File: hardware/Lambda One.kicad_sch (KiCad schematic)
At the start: 5 parts, among them IC1 01, SW1 SW_Push, U1 W65C816SxP, U3 ATF22V10C, Y1 TFT680

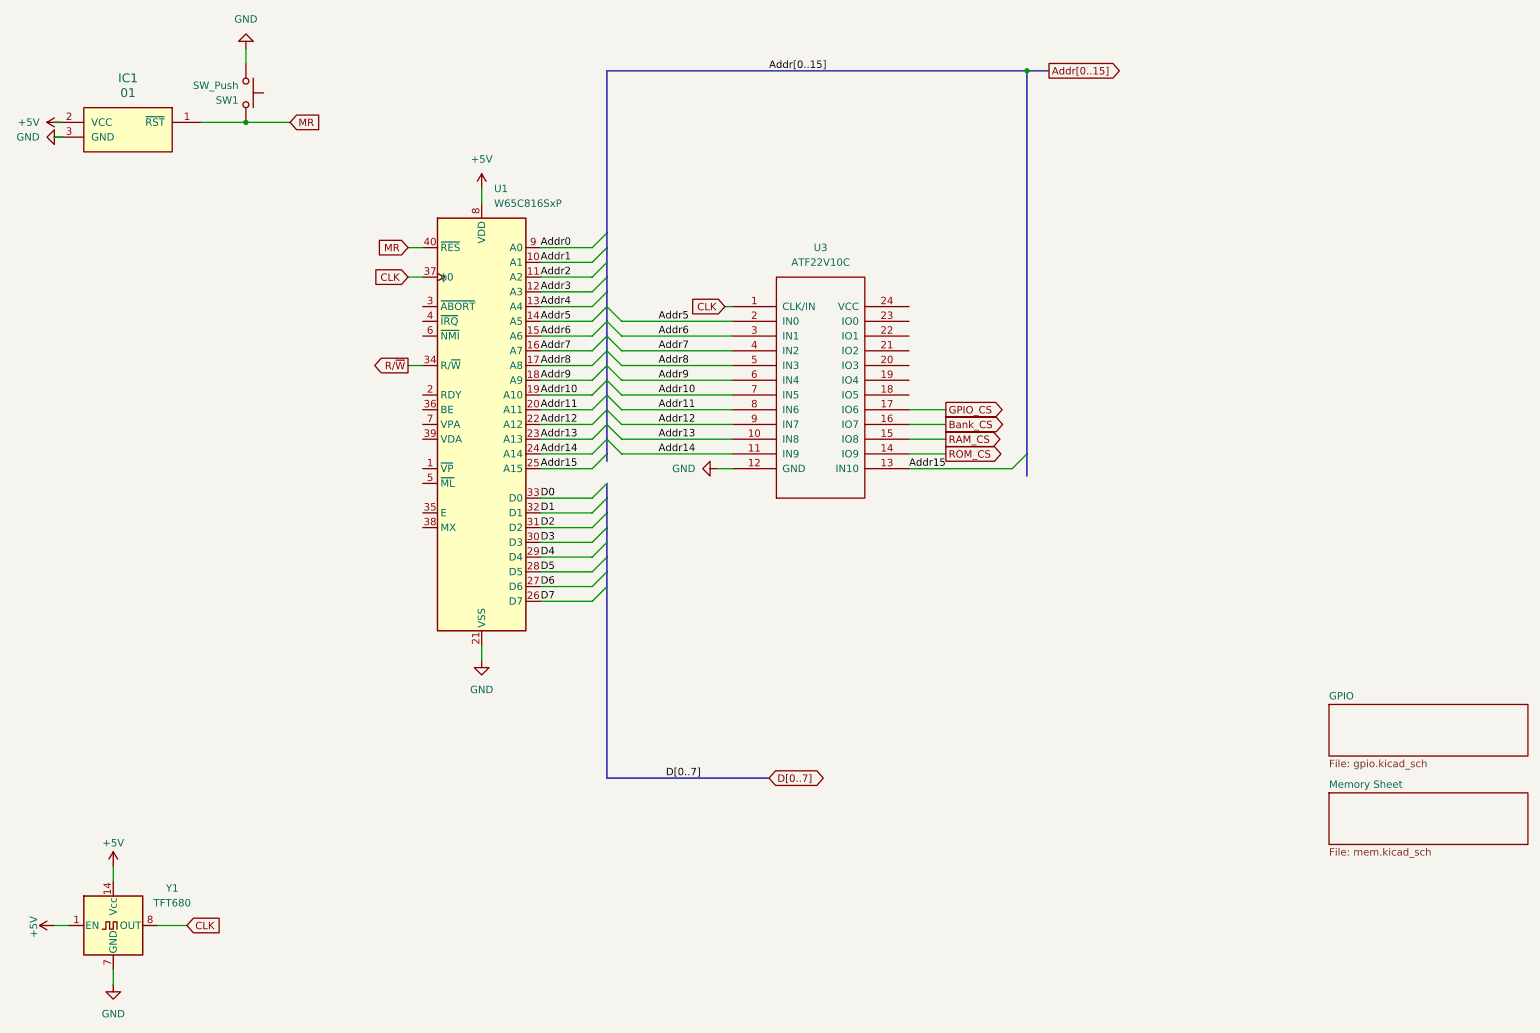
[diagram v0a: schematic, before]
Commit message: Improved labels
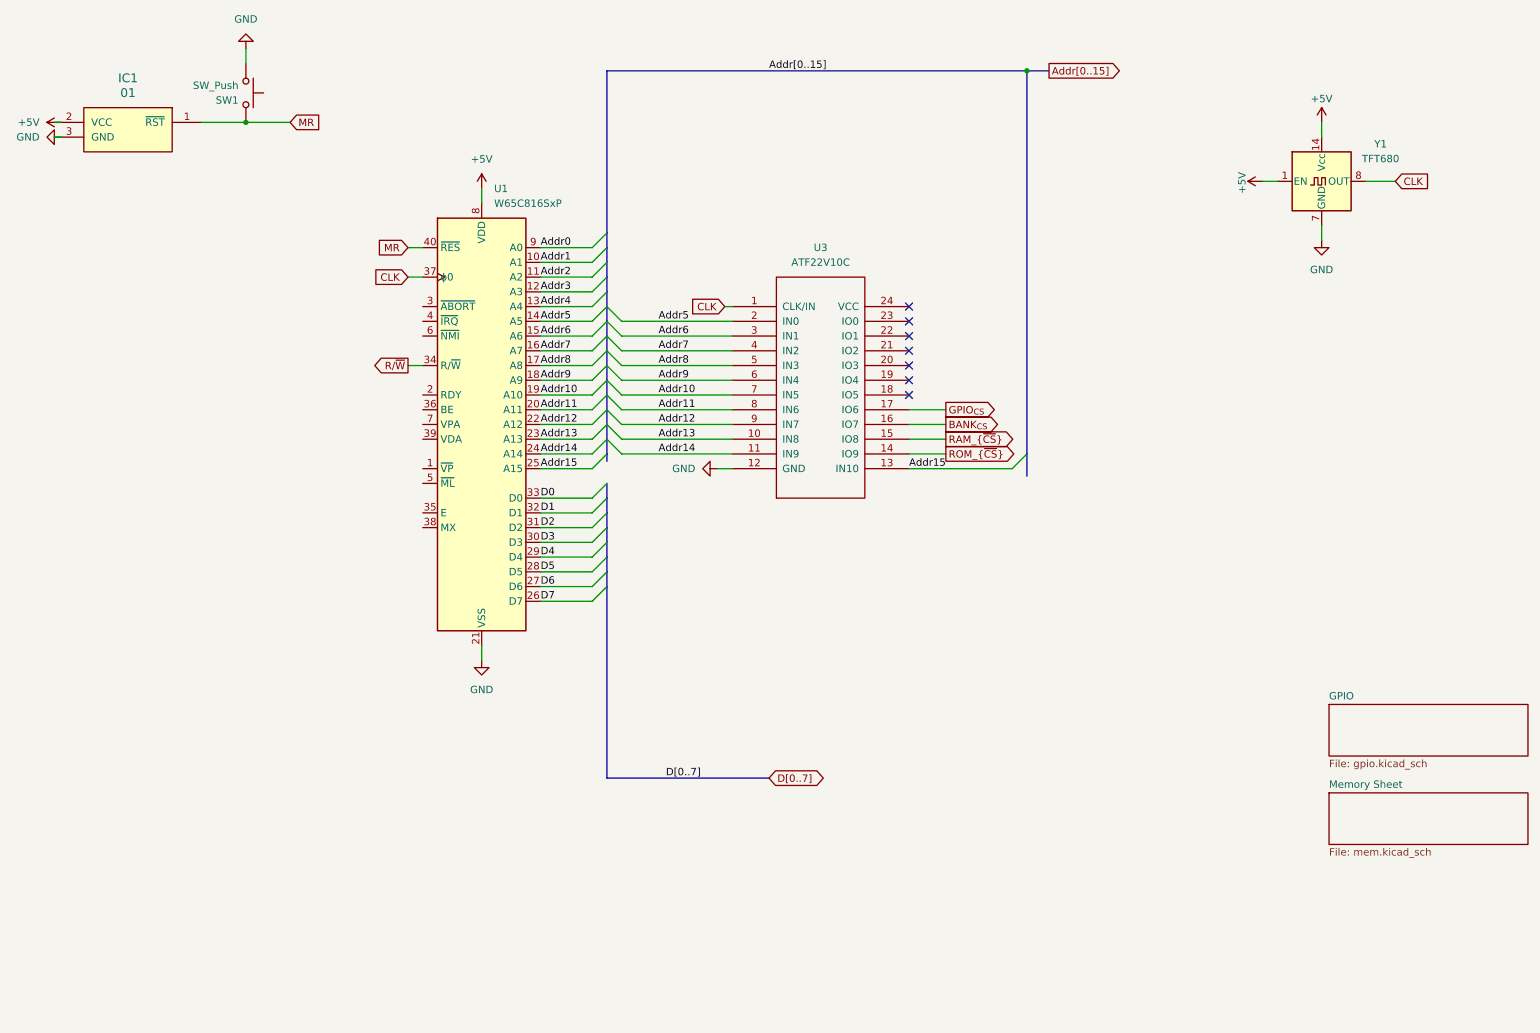
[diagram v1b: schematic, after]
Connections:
- net Bank_CS renamed BANK_{CS}
- net GPIO_CS renamed GPIO_{CS}
- net RAM_CS renamed RAM_{~{CS}}
- net ROM_CS renamed ROM_{~{CS}}
- no-connect marks 0 -> 7
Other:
- moved on the sheet: Y1
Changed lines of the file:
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@@
 		(color 0 0 0 0)
+	)
+	(no_connect
+		(at 175.26 69.85)
+	)
+	(no_connect
+		(at 175.26 72.39)
+	)
+	(no_connect
+		(at 175.26 77.47)
+	)
+	(no_connect
+		(at 175.26 82.55)
+	)
+	(no_connect
+		(at 175.26 85.09)
+	)
+	(no_connect
+		(at 175.26 80.01)
+	)
+	(no_connect
+		(at 175.26 74.93)
 	)
 	(bus_entry
@@
 	(wire
 		(pts
-			(xy 38.1 184.15) (xy 38.1 186.69)
+			(xy 246.38 55.88) (xy 246.38 58.42)
 		)
 		(stroke
@@
 	(wire
 		(pts
-			(xy 27.94 176.53) (xy 30.48 176.53)
+			(xy 236.22 48.26) (xy 238.76 48.26)
 		)
 		(stroke
@@
 	(wire
 		(pts
-			(xy 38.1 166.37) (xy 38.1 168.91)
+			(xy 246.38 38.1) (xy 246.38 40.64)
 		)
 		(stroke
@@
 	(wire
 		(pts
-			(xy 45.72 176.53) (xy 50.8 176.53)
+			(xy 254 48.26) (xy 259.08 48.26)
 		)
 		(stroke
@@
 	(global_label "CLK"
 		(shape input)
-		(at 50.8 176.53 0)
+		(at 259.08 48.26 0)
 		(fields_autoplaced yes)
 		(effects
@@
 		)
 		(property "Intersheetrefs" "${INTERSHEET_REFS}"
-			(at 57.3533 176.53 0)
+			(at 265.6333 48.26 0)
 			(effects
 				(font
@@
 		)
 	)
-	(global_label "ROM_CS"
+	(global_label "ROM_{~{CS}}"
 		(shape output)
 		(at 181.61 95.25 0)
@@
 		)
 		(property "Intersheetrefs" "${INTERSHEET_REFS}"
-			(at 192.0942 95.25 0)
+			(at 190.6815 95.25 0)
 			(effects
 				(font
@@
 		)
 	)
-	(global_label "Bank_CS"
+	(global_label "BANK_{CS}"
 		(shape output)
 		(at 181.61 90.17 0)
@@
 		)
 		(property "Intersheetrefs" "${INTERSHEET_REFS}"
-			(at 192.6384 90.17 0)
+			(at 191.5887 90.17 0)
 			(effects
 				(font
@@
 		)
 	)
-	(global_label "RAM_CS"
+	(global_label "RAM_{~{CS}}"
 		(shape output)
 		(at 181.61 92.71 0)
@@
 		)
 		(property "Intersheetrefs" "${INTERSHEET_REFS}"
-			(at 191.8523 92.71 0)
+			(at 190.4396 92.71 0)
 			(effects
 				(font
@@
 		)
 	)
-	(global_label "GPIO_CS"
+	(global_label "GPIO_{CS}"
 		(shape output)
 		(at 181.61 87.63 0)
@@
 		)
 		(property "Intersheetrefs" "${INTERSHEET_REFS}"
-			(at 192.5176 87.63 0)
+			(at 191.1049 87.63 0)
 			(effects
 				(font
@@
 	(symbol
 		(lib_id "power:+5V")
-		(at 27.94 176.53 90)
+		(at 236.22 48.26 90)
 		(unit 1)
 		(exclude_from_sim no)
@@
 		(dnp no)
 		(property "Reference" "#PWR020"
-			(at 31.75 176.53 0)
+			(at 240.03 48.26 0)
 			(effects
 				(font
@@
 		)
 		(property "Value" "+5V"
-			(at 24.384 176.784 0)
+			(at 232.664 48.514 0)
 			(effects
 				(font
@@
 		)
 		(property "Footprint" ""
-			(at 27.94 176.53 0)
+			(at 236.22 48.26 0)
 			(effects
 				(font
@@
 		)
 		(property "Datasheet" ""
-			(at 27.94 176.53 0)
+			(at 236.22 48.26 0)
 			(effects
 				(font
@@
 		)
 		(property "Description" "Power symbol creates a global label with name \"+5V\""
-			(at 27.94 176.53 0)
+			(at 236.22 48.26 0)
 			(effects
 				(font
@@
 	(symbol
 		(lib_id "power:+5V")
-		(at 38.1 166.37 0)
+		(at 246.38 38.1 0)
 		(unit 1)
 		(exclude_from_sim no)
@@
 		(dnp no)
 		(property "Reference" "#PWR014"
-			(at 38.1 170.18 0)
+			(at 246.38 41.91 0)
 			(effects
 				(font
@@
 		)
 		(property "Value" "+5V"
-			(at 38.1 162.306 0)
+			(at 246.38 34.036 0)
 			(effects
 				(font
@@
 		)
 		(property "Footprint" ""
-			(at 38.1 166.37 0)
+			(at 246.38 38.1 0)
 			(effects
 				(font
@@
 		)
 		(property "Datasheet" ""
-			(at 38.1 166.37 0)
+			(at 246.38 38.1 0)
 			(effects
 				(font
@@
 		)
 		(property "Description" "Power symbol creates a global label with name \"+5V\""
-			(at 38.1 166.37 0)
+			(at 246.38 38.1 0)
 			(effects
 				(font
@@
 	(symbol
 		(lib_id "Oscillator:TFT680")
-		(at 38.1 176.53 0)
+		(at 246.38 48.26 0)
 		(unit 1)
 		(exclude_from_sim no)
@@
 		(fields_autoplaced yes)
 		(property "Reference" "Y1"
-			(at 48.26 170.1098 0)
+			(at 256.54 41.8398 0)
 			(effects
 				(font
@@
 		)
 		(property "Value" "TFT680"
-			(at 48.26 172.6498 0)
+			(at 256.54 44.3798 0)
 			(effects
 				(font
@@
 		)
 		(property "Footprint" "Oscillator:Oscillator_DIP-14"
-			(at 49.53 185.42 0)
+			(at 257.81 57.15 0)
 			(effects
 				(font
@@
 		)
 		(property "Datasheet" "http://cdn-reichelt.de/documents/datenblatt/B400/OSZI.pdf"
-			(at 35.56 176.53 0)
+			(at 243.84 48.26 0)
 			(effects
 				(font
@@
 		)
 		(property "Description" "Crystal Clock Oscillator, DIP14-style metal package"
-			(at 38.1 176.53 0)
+			(at 246.38 48.26 0)
 			(effects
 				(font
@@
 	(symbol
 		(lib_id "power:GND")
-		(at 38.1 186.69 0)
+		(at 246.38 58.42 0)
 		(unit 1)
 		(exclude_from_sim no)
@@
 		(fields_autoplaced yes)
 		(property "Reference" "#PWR019"
-			(at 38.1 193.04 0)
+			(at 246.38 64.77 0)
 			(effects
 				(font
@@
 		)
 		(property "Value" "GND"
-			(at 38.1 191.77 0)
+			(at 246.38 63.5 0)
 			(effects
 				(font
@@
 		)
 		(property "Footprint" ""
-			(at 38.1 186.69 0)
+			(at 246.38 58.42 0)
 			(effects
 				(font
@@
 		)
 		(property "Datasheet" ""
-			(at 38.1 186.69 0)
+			(at 246.38 58.42 0)
 			(effects
 				(font
@@
 		)
 		(property "Description" "Power symbol creates a global label with name \"GND\" , ground"
-			(at 38.1 186.69 0)
-			(effects
-				(font
+			(at 246.38 58.42 0)
+			(effects
+				(font
